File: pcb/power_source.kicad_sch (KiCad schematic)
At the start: 5 parts, among them J4 USB_C_Receptacle_USB2.0_14P

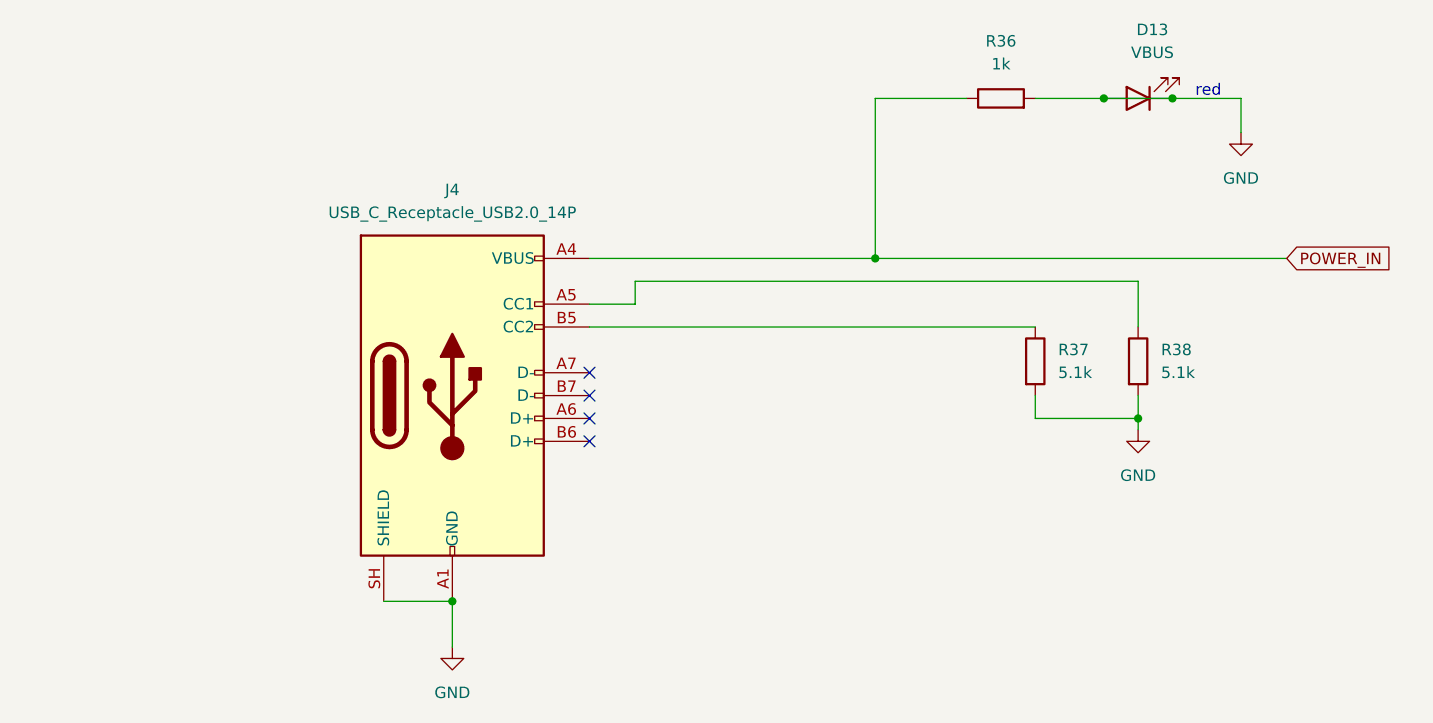
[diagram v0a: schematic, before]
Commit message: layout prep
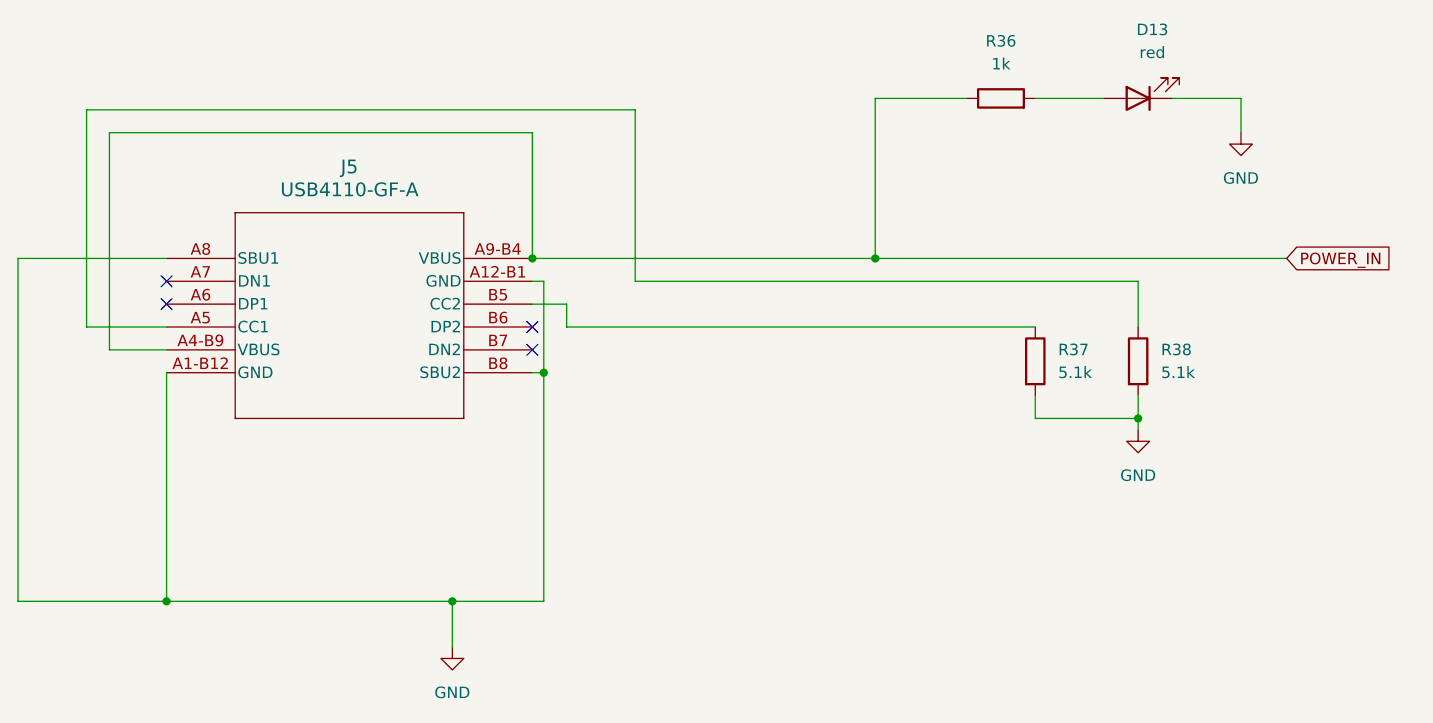
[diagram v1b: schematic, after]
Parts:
- removed J4: USB_C_Receptacle_USB2.0_14P, Package_DFN_QFN:WDFN-10-1EP_3x3mm_P0.5mm_EP1.8x2.5mm, symbol Connector:USB_C_Receptacle_USB2.0_14P
- added J5: USB4110-GF-A, USB4110_GF_A:USB4110-GF-A_GCT, symbol USB4110_GF_A:USB4110-GF-A
- D13: value VBUS -> red; footprint (none) -> LED_SMD:LED_0805_2012Metric_Pad1.15x1.40mm_HandSolder
- R36, R37, R38: footprint Resistor_THT:R_Array_SIP13 -> Resistor_SMD:R_0805_2012Metric_Pad1.20x1.40mm_HandSolder
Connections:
- net GND: now also J5.A1-B12 (GND), J5.A12-B1 (GND), J5.A8 (SBU1), J5.B8 (SBU2); no longer D13.2 (A), R36.2
- net POWER_IN: now also J5.A4-B9 (VBUS), J5.A9-B4 (VBUS)
- net at R38.1: now also J5.A5 (CC1)
- net at R37.1: now also J5.B5 (CC2)
- new net: D13.2 (A), R36.2
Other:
- note removed: "red"
